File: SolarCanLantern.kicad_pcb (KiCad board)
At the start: 2 copper layers, 43 x 22 mm, 16 parts, among them Q1 2N7002, Q2 2N7002, Q4 2N7002, SW1 SW_Push, U1 ATTINY13-20SSU

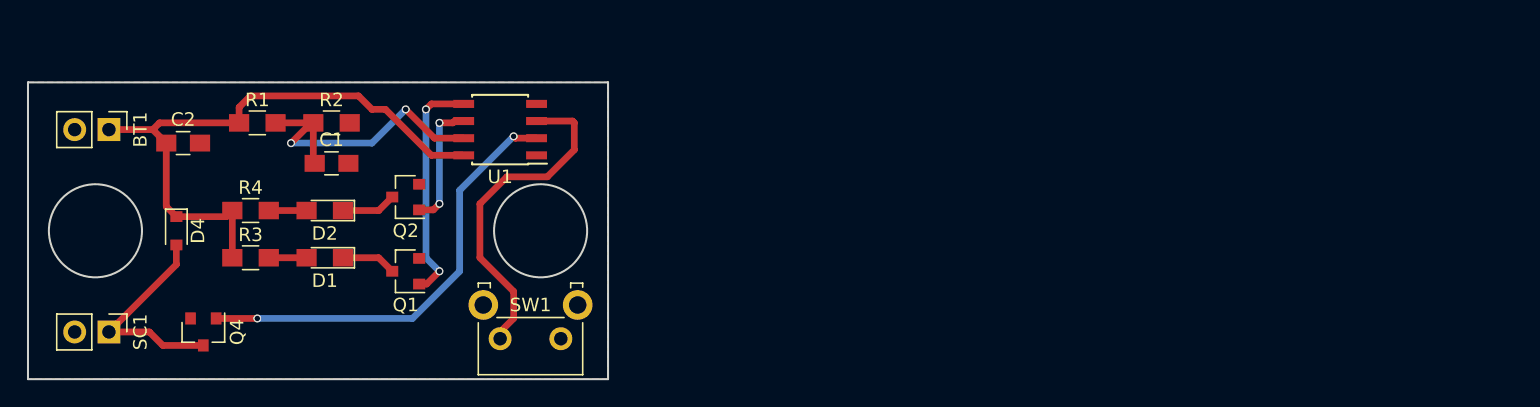
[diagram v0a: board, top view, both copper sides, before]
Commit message: got latest version from tejus and modified
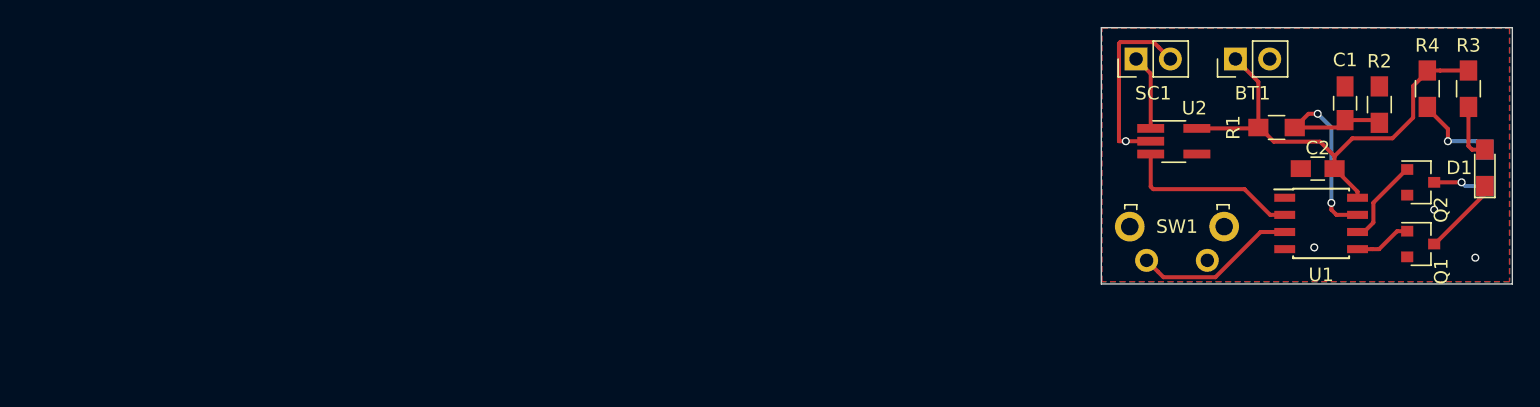
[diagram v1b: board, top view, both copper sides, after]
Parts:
- removed D4: D, Diodes_SMD:D_0805
- removed Q4: 2N7002, TO_SOT_Packages_SMD:SOT-23
- added U2: MAX40200, TO_SOT_Packages_SMD:TSOT-23-5_HandSoldering, F.Cu at (202.4, 86.4)
- D2: moved to B.Cu
- moved R3 91.1 mm to (224.3, 82.5), turned to 270 degrees
- moved R4 87.7 mm to (221.2, 82.5), turned to 270 degrees
- moved D1 86.3 mm to (225.5, 88.3), turned to 90 degrees
- moved D2 86.1 mm to (225.5, 88.3), turned to 90 degrees
- moved C2 84.1 mm to (213.1, 88.4), turned to 180 degrees
- moved BT1 83.7 mm to (207.0, 80.3), turned to 90 degrees
- moved SC1 78.8 mm to (199.6, 80.3), turned to 90 degrees
- moved R2 77.7 mm to (217.7, 83.6), turned to 90 degrees
- moved R1 75.6 mm to (210.1, 85.3)
- moved C1 75.3 mm to (215.1, 83.5), turned to 90 degrees
- moved Q1 75.3 mm to (220.7, 94.0), turned to 0 degrees
- moved Q2 75.2 mm to (220.7, 89.4), turned to 0 degrees
- moved U1 61.3 mm to (213.4, 92.5), turned to 0 degrees
- moved SW1 48.3 mm to (204.9, 95.2)
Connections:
- SC1 pad 1: Net-(D4-Pad2) -> /SolarIn
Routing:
- net /~SOLAR: track 32.9 -> 13.2 mm, vias 2 -> 0
- net Net-(D4-Pad2): track 15.9 -> 0.00 mm
- net GND: track 0.00 -> 14.0 mm, vias 0 -> 4
- net /LEDA: track 17.3 -> 4.23 mm, vias 2 -> 0
- net /Switch: track 25.0 -> 12.1 mm
- net +BATT: track 44.8 -> 34.7 mm
- net /SolarIn: track 0.00 -> 5.60 mm
- net /VBatt_Divider: track 22.8 -> 18.3 mm
- net Net-(D2-Pad2): track 2.80 -> 6.17 mm, vias 0 -> 1
- net /LEDB: track 9.54 -> 6.47 mm, vias 2 -> 0
- net Net-(D1-Pad1): track 4.06 -> 5.88 mm
- net Net-(D1-Pad2): track 2.80 -> 4.22 mm
- net Net-(D2-Pad1): track 4.06 -> 3.87 mm, vias 0 -> 1
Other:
- board size 43 x 22 mm -> 30.5 x 19 mm
- net class Default: clearance 0.2 -> 0.25; trace_width 0.5 -> 0.3
- rule pad_to_mask_clearance: 0.2 -> 0
- rule trace_clearance: 0.2 -> 0.25
- board text added: "Haiti Solar Lights Project Tejus Rao and Erik Meike 2018"
- board text removed: "HMC Haiti Solar Lights Project 2018 PCB Rev. 2"
